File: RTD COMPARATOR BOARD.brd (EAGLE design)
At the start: 94 x 80 mm, 50 parts, among them IC1 LM324N, IC2 LM324N, IC3 LM324N, IC4 LM324N, IC5 LM324N, IC6 LM324N, IC7 LM324N, IC8 LM324N, IC9 LM324N, X1 5566-10, X2 5566-6

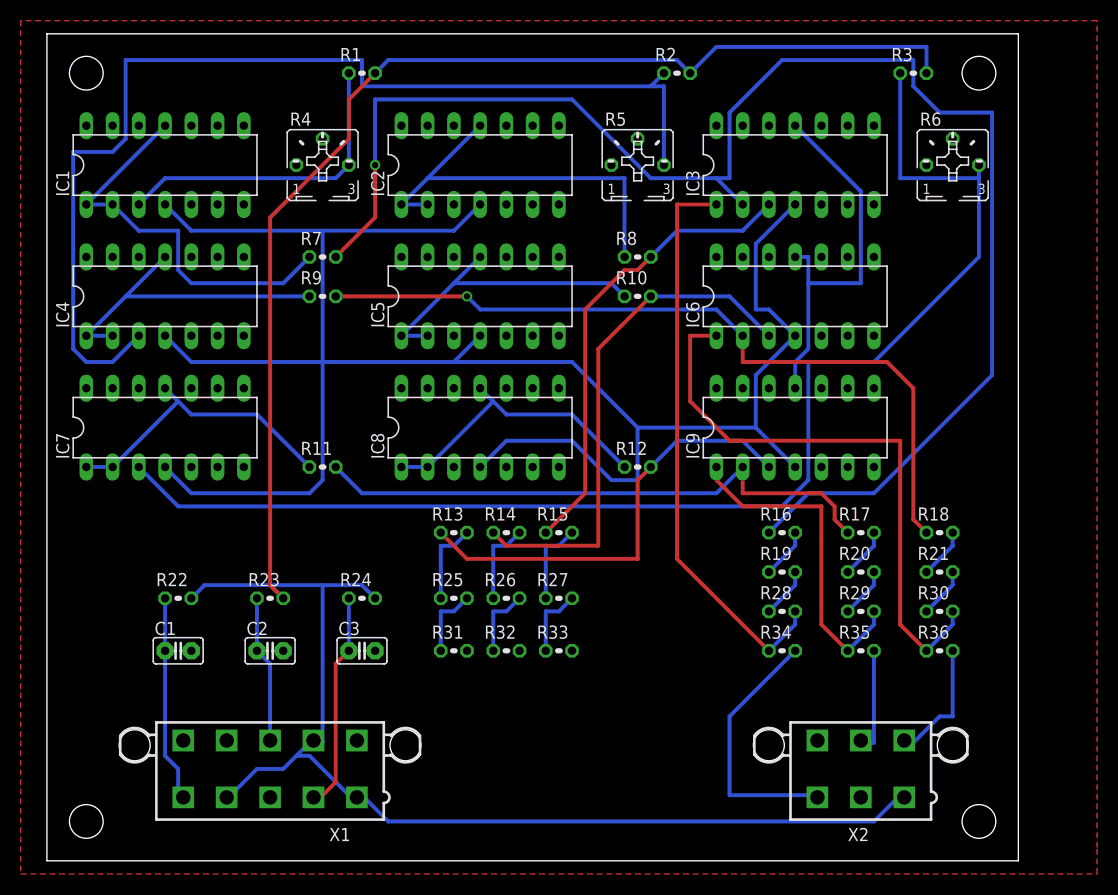
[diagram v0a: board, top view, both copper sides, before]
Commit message: 4th commit
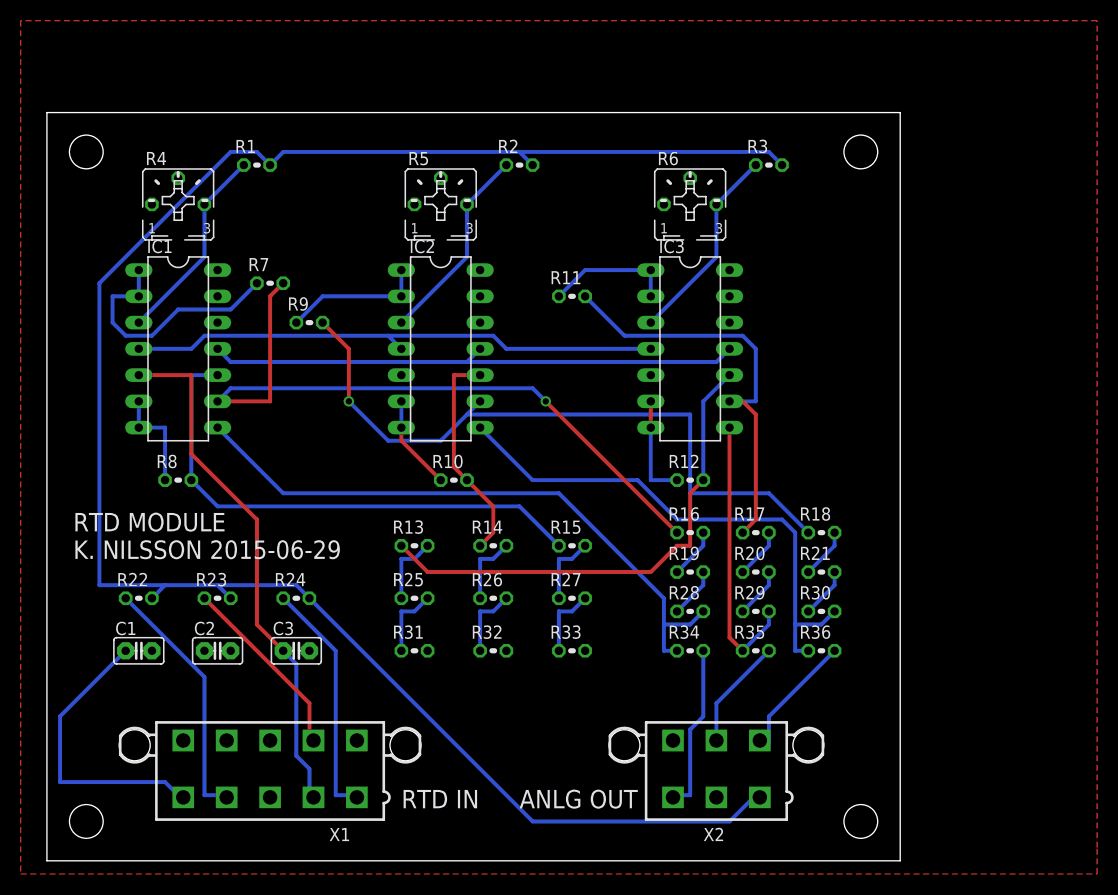
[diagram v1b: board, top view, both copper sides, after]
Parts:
- removed IC4, IC5, IC6, IC7, IC8, IC9: LM324N, linear:DIL14
- R22, R23, R24: value 1k -> 10k
- R34: value 220 -> 220k
- moved R8 49.4 mm to (12.7, 36.8)
- moved R11 29.2 mm to (50.8, 54.6)
- moved R6 25.7 mm to (62.2, 63.5)
- moved R10 25.1 mm to (39.4, 36.8)
- moved IC3 20.5 mm to (62.2, 49.5), turned to 270 degrees
- moved R5 19.4 mm to (38.1, 63.5)
- moved IC2 18.2 mm to (38.1, 49.5), turned to 270 degrees
- moved IC1 17.8 mm to (12.7, 49.5), turned to 270 degrees
- moved R2 17.6 mm to (45.7, 67.3)
- moved R3 16.6 mm to (69.8, 67.3)
- moved R4 14.5 mm to (12.7, 63.5)
- moved X2 14.0 mm to (64.8, 8.89)
- moved R1 13.5 mm to (20.3, 67.3)
- moved R18 11.4 mm to (74.9, 31.8)
- moved R21 11.4 mm to (74.9, 27.9)
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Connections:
- new net N$11: R23.1, X1.7
- new net N$3: R24.1, X1.1
- net N$10: now also IC2.3; no longer IC4.3
- net N$14: no longer R22.1
- net N$15: now also IC2.1, IC2.2; no longer IC4.1, IC4.11, IC4.2
- net N$16: now also IC2.9; no longer IC6.2
- net N$18: now also IC1.9; no longer IC3.2
- net N$19: no longer IC1.11
- net N$20: now also IC2.6, IC2.7; no longer IC5.1, IC5.11, IC5.2
- net N$21: now also IC1.6, IC1.7; no longer IC2.1, IC2.11, IC2.2
- net N$22: now also IC1.10; no longer IC3.3
- net N$23: now also IC1.8; no longer IC3.1
- net N$24: now also C3.1, IC1.5, X1.2; no longer IC2.3
- net N$25: no longer C2.1, R23.1
- net N$26: now also IC2.10; no longer IC6.3
- net N$29: now also IC2.8; no longer IC6.1
- net N$32: now also IC3.5; no longer IC8.3
- net N$33: now also IC3.3; no longer IC7.3
- net N$34: now also IC3.1, IC3.2; no longer IC7.1, IC7.11, IC7.2
- net N$35: now also IC3.9; no longer IC9.2
- net N$36: now also IC3.6, IC3.7; no longer IC8.1, IC8.11, IC8.2
- net N$37: now also IC3.10; no longer IC9.3
- net N$38: now also IC3.8; no longer IC9.1
- net N$4: now also R22.1, X1.4; no longer C3.1, R24.1, X1.2
- net N$9: now also IC2.5; no longer IC5.3
- net V+: no longer IC4.4, IC5.4, IC6.4, IC7.4, IC8.4, IC9.4
- net V-: now also IC1.11, IC2.11; no longer IC6.11, IC9.11
- net VCC: no longer X1.1, X1.4, X1.7
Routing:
- net V+: track 193.4 -> 52.4 mm
- net N$33: track 126.2 -> 19.4 mm
- net N$10: track 104.2 -> 19.4 mm
- net N$18: track 148.6 -> 67.8 mm
- net N$24: track 0.00 -> 50.9 mm
- net VCC: track 223.5 -> 181.9 mm
- net N$21: track 40.0 -> 10.2 mm
- net N$26: track 49.9 -> 21.2 mm
- net N$3: track 0.00 -> 23.2 mm
- net N$20: track 30.4 -> 9.20 mm
- net N$11: track 0.00 -> 18.6 mm
- net N$36: track 28.6 -> 10.2 mm
- net N$15: track 31.1 -> 13.8 mm
- net N$34: track 28.6 -> 12.5 mm
- net N$35: track 56.5 -> 41.3 mm
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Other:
- board size 94 x 80 mm -> 82.5 x 72.4 mm
- board text added: "ANLG OUT"
- board text added: "RTD IN"
- board text added: "RTD MODULE K. NILSSON 2015-06-29"
